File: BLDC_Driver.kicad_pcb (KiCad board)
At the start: 2 copper layers, 65.1 x 63 mm, 117 parts, among them J1 Conn_01x05, J10 Conn_01x01, J2 Conn_01x05, J4 USB_C_Receptacle_USB2.0_14P, J5 CAN, J6 Conn_01x01, J7 Conn_01x01, J8 Conn_01x01, J9 Conn_01x01, Q1 NMOS, Q2 NMOS, Q3 NMOS, Q4 NMOS, Q5 NMOS, Q6 NMOS, SW1 SW_Push, U1 STSPIN32G4, U3 ST1S14PHR, U4 TCAN330G, Y1 Crystal_GND24_Small

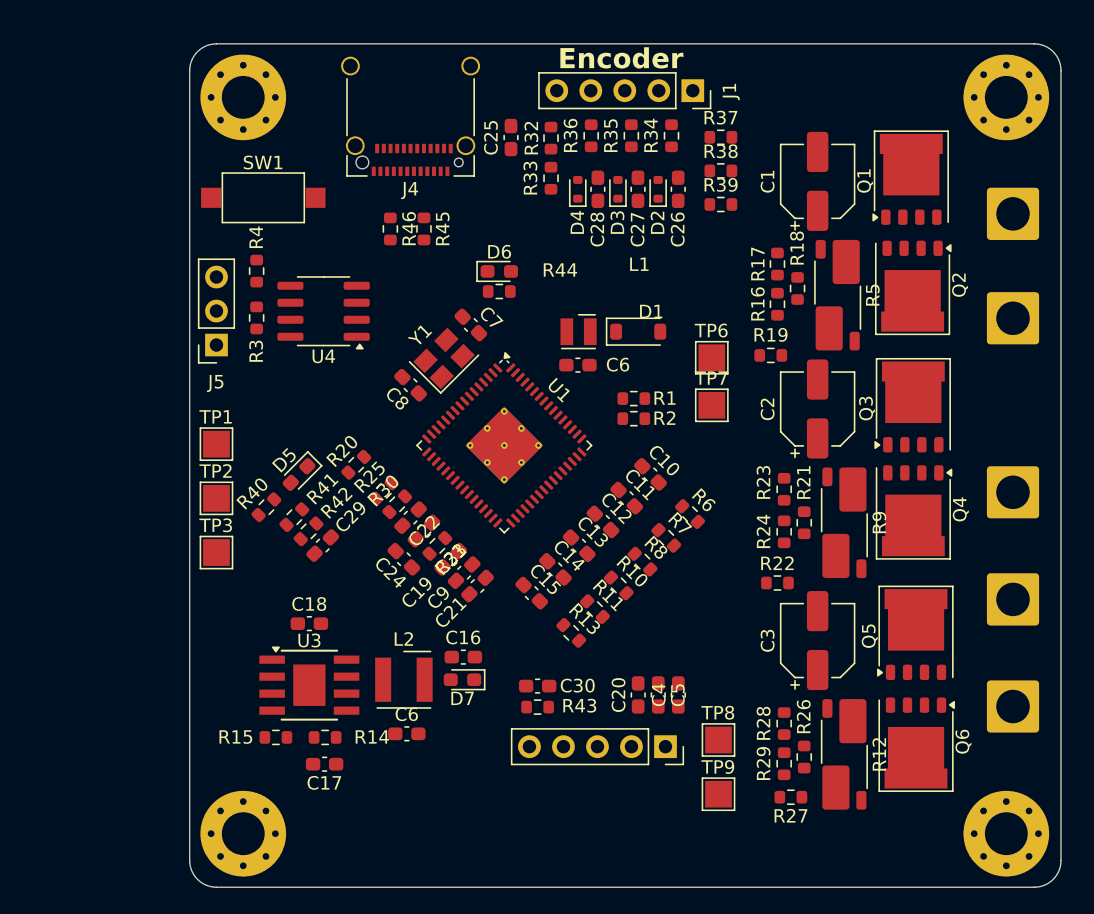
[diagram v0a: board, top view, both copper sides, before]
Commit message: All DONE >?git add .git add .
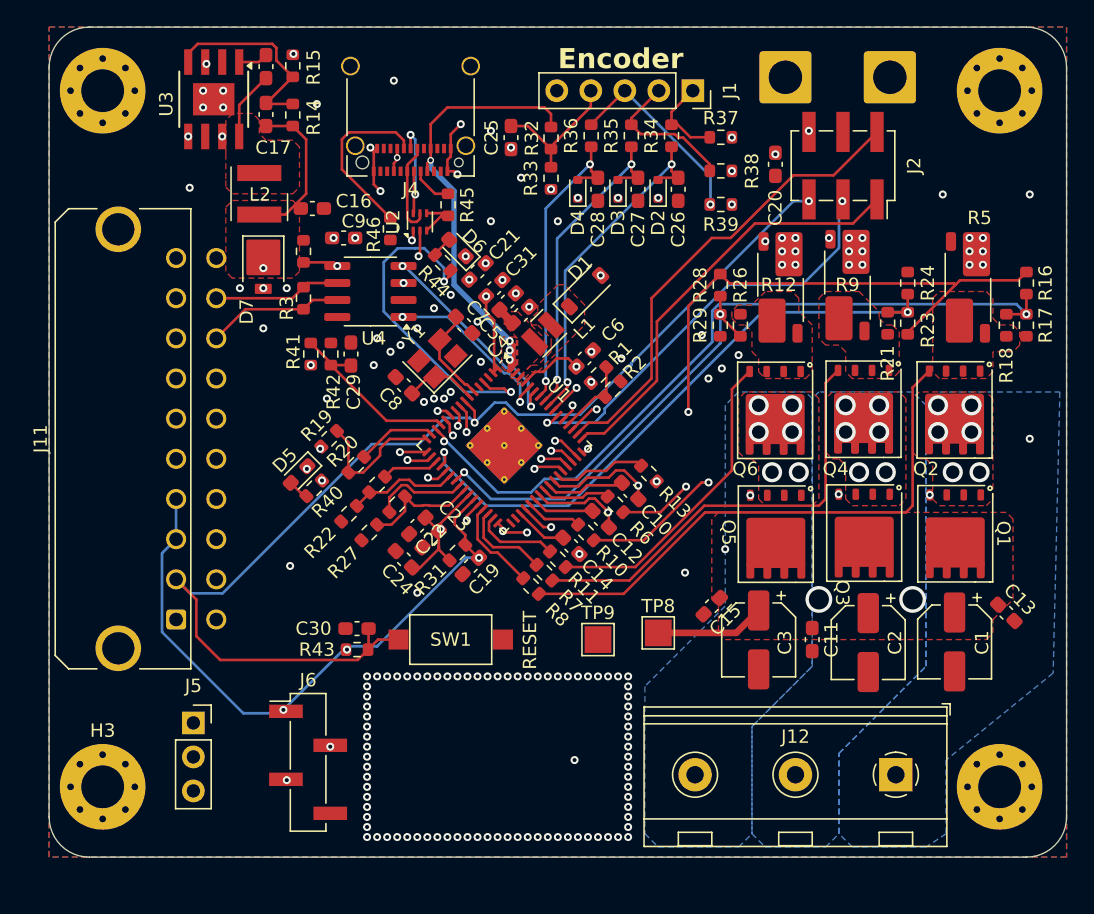
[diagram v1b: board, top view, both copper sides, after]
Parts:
- removed the C6 at (221.7, 125.0)
- removed J10, J9: Conn_01x01, Connector_Wire:SolderWire-2sqmm_1x01_D2mm_OD3.9mm
- removed TP1, TP2, TP3, TP6, TP7: TestPoint, TestPoint:TestPoint_Pad_2.0x2.0mm
- added C31: 100n, Capacitor_SMD:C_0603_1608Metric_Pad1.08x0.95mm_HandSolder, F.Cu at (228.2, 91.8)
- added J11: Conn_02x10_Counter_Clockwise, Connector_Molex:Molex_Micro-Fit_3.0_43045-2021_2x10-1MP_P3.00mm_Horizontal, F.Cu at (204.5, 116.5)
- added J12: Screw_Terminal_01x03, TerminalBlock_RND:TerminalBlock_RND_205-00068_1x03_P7.50mm_Horizontal, F.Cu at (258.2, 128.1)
- added U2: ECMF02-2AMX6, Package_DFN_QFN:ST_UQFN-6L_1.5x1.7mm_P0.5mm, F.Cu at (222.7, 86.8)
- D7: value D -> ESH2PB; footprint Diode_SMD:D_0603_1608Metric_Pad1.05x0.95mm_HandSolder -> Diode_SMD:D_SMP_DO-220AA
- J2: value Conn_01x05 -> Conn_02x03_Counter_Clockwise; footprint Connector_PinSocket_2.54mm:PinSocket_1x05_P2.54mm_Vertical -> Connector_PinSocket_2.54mm:PinSocket_2x03_P2.54mm_Vertical_SMD
- J6: value Conn_01x01 -> Conn_01x04; footprint Connector_Wire:SolderWire-2sqmm_1x01_D2mm_OD3.9mm -> Connector_PinHeader_2.54mm:PinHeader_1x04_P2.54mm_Vertical_SMD_Pin1Left
- Q1, Q2, Q3, Q4, Q5, Q6: value NMOS -> STL160N10F8; footprint Package_DFN_QFN:PQFN-8-EP_6x5mm_P1.27mm_Generic -> PCM_Package_SON_AKL:Infineon_PG-TDSON-8
- moved J6 56.4 mm to (214.3, 127.2), turned to 0 degrees
- moved R15 50.2 mm to (213.2, 75.1), turned to 90 degrees
- moved C17 48.7 mm to (211.2, 78.8), turned to 90 degrees
- moved R14 46.6 mm to (213.2, 78.8), turned to 90 degrees
- moved J2 45.4 mm to (254.3, 82.6)
- moved U3 44.3 mm to (207.3, 77.6), turned to -90 degrees
- moved C18 41.7 mm to (211.2, 75.2), turned to -90 degrees
- moved C20 40.9 mm to (249.2, 82.5), turned to -90 degrees
- moved L2 37.9 mm to (210.7, 84.7), turned to -90 degrees
- moved R27 37.2 mm to (218.9, 110.0), turned to 45 degrees
- moved C1 35.9 mm to (262.6, 118.2), turned to -90 degrees
- moved SW1 35.8 mm to (225.0, 118.0), turned to 180 degrees
- moved C16 35.4 mm to (214.7, 85.8)
- moved R12 35.2 mm to (249.6, 91.7), turned to 90 degrees
- moved D7 34.3 mm to (211.0, 90.1), turned to -90 degrees
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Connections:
- net /Connectivity/CAN_H renamed CAN_H
- net /Connectivity/CAN_L renamed CAN_L
- C16 pad 1: Net-(D7-A) -> 5V
- C17 pad 1: Net-(D7-A) -> 5V
- D7 pad 2: Net-(D7-A) -> GND
- J2 pad 1: 3V3 -> /Connectivity/SWDIO
- J2 pad 3: /Connectivity/SWDIO -> /Connectivity/SWO
- J2 pad 4: /Connectivity/nRST -> GND
- J2 pad 5: GND -> /Connectivity/nRST
- J4 pad A6: /Connectivity/USB_DP -> /Connectivity/USB_DP_Conn
- J4 pad A7: /Connectivity/USB_DM -> /Connectivity/USB_DM_Conn
- J4 pad B6: /Connectivity/USB_DP -> /Connectivity/USB_DP_Conn
- J4 pad B7: /Connectivity/USB_DM -> /Connectivity/USB_DM_Conn
- J6 pad 1: /OUT1 -> 3V3
- L2 pad 2: Net-(D7-A) -> 5V
- Q1 pad 1: VM -> /OUT1
- Q1 pad 2: Net-(Q1-G) -> /OUT1
- Q1 pad 4: (no net) -> Net-(Q1-G)
- Q1 pad 5: (no net) -> VM
- Q2 pad 1: /OUT1 -> /H-Bridge/VSHUNT1P
- Q2 pad 2: Net-(Q2-G) -> /H-Bridge/VSHUNT1P
- Q2 pad 3: Net-(Q2-S) -> /H-Bridge/VSHUNT1P
- Q2 pad 4: (no net) -> Net-(Q2-G)
- Q2 pad 5: (no net) -> /OUT1
- Q3 pad 1: VM -> /OUT2
- Q3 pad 2: Net-(Q3-G) -> /OUT2
- Q3 pad 4: (no net) -> Net-(Q3-G)
- Q3 pad 5: (no net) -> VM
- Q4 pad 1: /OUT2 -> /H-Bridge/VSHUNT2P
- Q4 pad 2: Net-(Q4-G) -> /H-Bridge/VSHUNT2P
- Q4 pad 3: Net-(Q4-S) -> /H-Bridge/VSHUNT2P
- Q4 pad 4: (no net) -> Net-(Q4-G)
- Q4 pad 5: (no net) -> /OUT2
- Q5 pad 1: VM -> /OUT3
- Q5 pad 2: Net-(Q5-G) -> /OUT3
- Q5 pad 4: (no net) -> Net-(Q5-G)
- Q5 pad 5: (no net) -> VM
- Q6 pad 1: /OUT3 -> /H-Bridge/VSHUNT3P
- Q6 pad 2: Net-(Q6-G) -> /H-Bridge/VSHUNT3P
- Q6 pad 3: Net-(Q6-S) -> /H-Bridge/VSHUNT3P
- Q6 pad 4: (no net) -> Net-(Q6-G)
- Q6 pad 5: (no net) -> /OUT3
- R12 pad 1: Net-(Q6-S) -> /H-Bridge/VSHUNT3P
- R12 pad 3: /H-Bridge/VSHUNT3N -> GND
- R14 pad 1: Net-(D7-A) -> 5V
- R19 pad 1: /H-Bridge/VSHUNT1N -> GND
- R22 pad 1: /H-Bridge/VSHUNT2N -> GND
- R27 pad 1: /H-Bridge/VSHUNT3N -> GND
- R5 pad 1: Net-(Q2-S) -> /H-Bridge/VSHUNT1P
- R5 pad 3: /H-Bridge/VSHUNT1N -> GND
- R9 pad 1: Net-(Q4-S) -> /H-Bridge/VSHUNT2P
- R9 pad 3: /H-Bridge/VSHUNT2N -> GND
- U1 pad 10: unconnected-(U1-PC1-Pad10) -> /MCU/PC1
- U1 pad 11: unconnected-(U1-PC2-Pad11) -> /MCU/PC2
- U1 pad 12: unconnected-(U1-PC3-Pad12) -> /MCU/PC3
- U1 pad 21: unconnected-(U1-PC4-Pad21) -> /MCU/PC4
- U1 pad 28: unconnected-(U1-PB10-Pad28) -> /MCU/PB10
- U1 pad 3: unconnected-(U1-PC13-Pad3) -> /MCU/PC13
- U1 pad 47: /MCU/USB_DM -> /Connectivity/USB_DM
- U1 pad 48: /MCU/USB_DP -> /Connectivity/USB_DP
- U1 pad 5: unconnected-(U1-PC15-Pad5) -> /MCU/PC15
- U1 pad 51: unconnected-(U1-PA15-Pad51) -> /MCU/PA15
- U1 pad 53: unconnected-(U1-PD2-Pad53) -> /MCU/PD2
- U1 pad 55: unconnected-(U1-PB4-Pad55) -> /MCU/PB4
- U1 pad 9: unconnected-(U1-PC0-Pad9) -> /MCU/PC0
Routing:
- net /Connectivity/nRST: track 0.00 -> 85.8 mm, vias 0 -> 2
- net VREF+: track 0.00 -> 72.9 mm, vias 0 -> 2
- net /MCU/OPP1: track 0.00 -> 56.7 mm, vias 0 -> 2
- net CAN_L: track 0.00 -> 55.8 mm
- net 3V3: track 0.00 -> 53.5 mm, vias 0 -> 17
- net CAN_H: track 0.00 -> 52.4 mm
- net /MCU/PB4: track 0.00 -> 49.2 mm, vias 0 -> 1
- net 5V: track 0.00 -> 48.0 mm, vias 0 -> 6
- net /MCU/OPP2: track 0.00 -> 46.8 mm, vias 0 -> 2
- net /MCU/PB10: track 0.00 -> 44.9 mm, vias 0 -> 1
- net /Connectivity/UART_RX: track 0.00 -> 43.7 mm, vias 0 -> 2
- net Net-(Q2-G): track 0.00 -> 41.2 mm
- net /MCU/PD2: track 0.00 -> 39.4 mm, vias 0 -> 1
- net /Connectivity/UART_TX: track 0.00 -> 36.6 mm, vias 0 -> 2
- net /MCU/PC4: track 0.00 -> 35.7 mm, vias 0 -> 1
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- added copper zone on F.Cu, net /H-Bridge/VSHUNT1P
- added copper zone on F.Cu, net /H-Bridge/VSHUNT2P
- added copper zone on F.Cu, net /H-Bridge/VSHUNT3P
- added copper zone on F.Cu, net /MCU/SW
- added copper zone on B.Cu, net /OUT1
- added copper zone on F.Cu, net /OUT1
- added copper zone on B.Cu, net /OUT2
- added copper zone on F.Cu, net /OUT2
- added copper zone on B.Cu, net /OUT3
- added copper zone on F.Cu, net /OUT3
- added copper zone on In4.Cu, net 3V3
- added copper zone on F.Cu, net 5V
- added copper zone on In2.Cu, net 5V
- added copper zone on B.Cu, net GND
- added copper zone on F.Cu, net GND
- added copper zone on In1.Cu, net GND
- added copper zone on In3.Cu, net GND
- added copper zone on F.Cu, net Net-(U3-SW)
- added copper zone on F.Cu, net VCC
- added copper zone on F.Cu, net VM
- added copper zone on In2.Cu, net VM
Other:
- board size 65.1 x 63 mm -> 76 x 62 mm
- copper layers 2 -> 6
- board text added: "RESET"
